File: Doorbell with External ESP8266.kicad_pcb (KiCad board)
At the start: 4 copper layers, 76.2 x 50.8 mm, 29 parts, among them J101 Transformer, J102 To Rectifier, J103 From Rectifier, J104 Button, J105 Chime, K102 Relay, Q101 Q_NMOS_GSD, U101 WeMos_D1_mini, U102 EL817, U104 XC6220B331MR-G

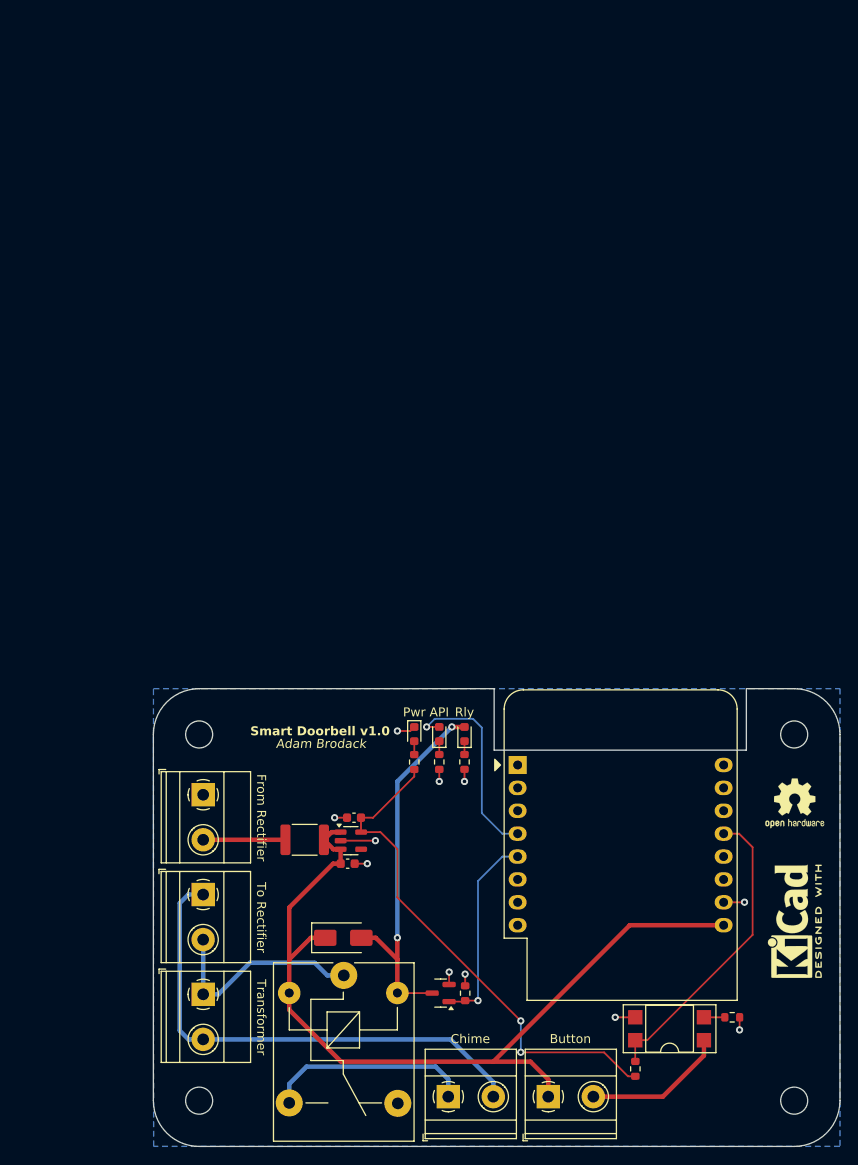
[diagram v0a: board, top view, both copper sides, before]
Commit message: Updated schematic & PCB
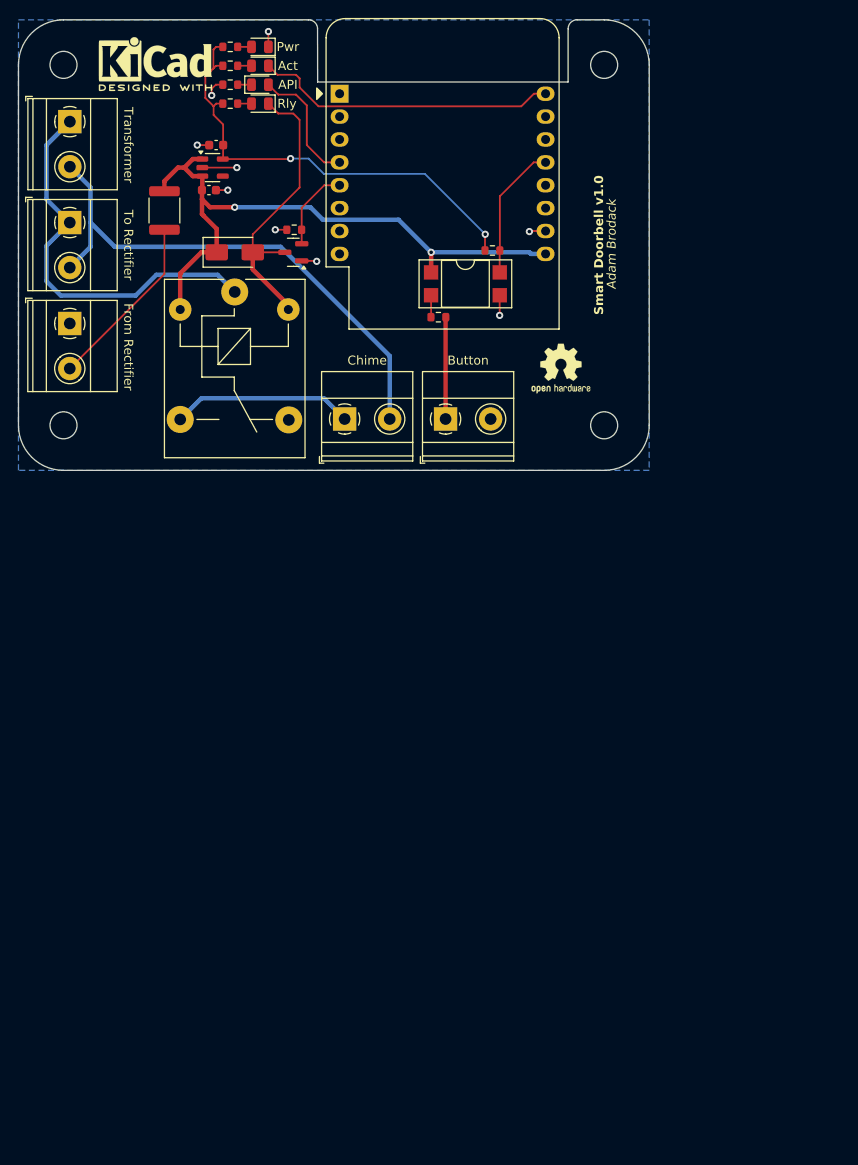
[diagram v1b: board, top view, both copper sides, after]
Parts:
- removed C105: 22uF, Capacitor_SMD:C_0603_1608Metric
- removed C106: 4.7uF, Capacitor_SMD:C_0603_1608Metric
- removed D106: Yellow, LED_SMD:LED_0603_1608Metric
- removed K102: Relay, Relay_THT:Relay_SPDT_SANYOU_SRD_Series_Form_C
- removed R108: 10K, Resistor_SMD:R_0603_1608Metric
- removed U104: XC6220B331MR-G, Package_TO_SOT_SMD:SOT-23-5
- added C101: 22uF, Capacitor_SMD:C_0603_1608Metric, F.Cu at (41.1, 38.9)
- added C102: 4.7uF, Capacitor_SMD:C_0603_1608Metric, F.Cu at (41.9, 33.9)
- added D102: Green, LED_SMD:LED_0805_2012Metric, F.Cu at (46.8, 27.2)
- added D103: Yellow, LED_SMD:LED_0805_2012Metric, F.Cu at (46.8, 25.1)
- added K101: Relay, Relay_THT:Relay_SPDT_SANYOU_SRD_Series_Form_C, F.Cu at (44.0, 50.2)
- added R105: 10K, Resistor_SMD:R_0603_1608Metric, F.Cu at (50.6, 43.3)
- added R107: 10K, Resistor_SMD:R_0603_1608Metric, F.Cu at (72.6, 45.6)
- added U103: EL817, Package_DIP:DIP-4_W7.62mm_SMDSocket_SmallPads, F.Cu at (69.6, 49.3)
- D101: value D_Small -> Red; footprint Diode_SMD:D_SMA -> LED_SMD:LED_0805_2012Metric
- D104: value Red -> White; footprint LED_SMD:LED_0603_1608Metric -> LED_SMD:LED_0805_2012Metric
- D105: value Green -> D_Small; footprint LED_SMD:LED_0603_1608Metric -> Diode_SMD:D_SMA
- J102: value To Rectifier -> From Rectifier
- J103: value From Rectifier -> To Rectifier
- J104: value Button -> Chime
- J105: value Chime -> Button
- R104: value 10K -> 1K
- U102: value EL817 -> XC6220B331MR-G; footprint Package_DIP:DIP-4_W7.62mm_SMDSocket_SmallPads -> Package_TO_SOT_SMD:SOT-23-5
- moved REF** 118.7 mm to (35.2, 24.9), turned to 0 degrees
- moved U102 108.2 mm to (41.5, 36.4), turned to 0 degrees
- moved R104 102.1 mm to (43.5, 29.3), turned to 180 degrees
- moved D101 99.3 mm to (46.8, 23.0), turned to 180 degrees
- moved J101 98.0 mm to (25.7, 31.3)
- moved R106 84.3 mm to (66.6, 53.0), turned to 180 degrees
- moved Q101 83.8 mm to (50.5, 45.8)
- moved R101 82.0 mm to (43.5, 23.0), turned to 180 degrees
- moved R103 81.5 mm to (43.5, 25.1), turned to 180 degrees
- moved R102 78.7 mm to (43.5, 27.2), turned to 0 degrees
- moved J104 78.5 mm to (56.2, 64.3)
- moved H104 77.9 mm to (85.0, 65.0)
- moved H102 77.2 mm to (85.0, 25.0)
- moved U101 77.1 mm to (55.6, 28.2)
- moved H103 76.4 mm to (25.0, 65.0)
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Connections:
- D101 pad 1: VCC -> GND
- D101 pad 2: /RELAY_LED -> Net-(D101-A)
- D104 pad 1: GND -> /RELAY_LED
- D105 pad 1: Net-(D105-K) -> VCC
- D105 pad 2: /HA_STATUS -> /RELAY_LED
- F101 pad 1: Net-(J103-Pin_2) -> Net-(J102-Pin_2)
- J102 pad 1: /AC_B -> GND
- J102 pad 2: /AC_A -> Net-(J102-Pin_2)
- J103 pad 1: GND -> /AC_A
- J103 pad 2: Net-(J103-Pin_2) -> /AC_B
- J104 pad 1: VCC -> Net-(J104-Pin_1)
- J104 pad 2: Net-(J104-Pin_2) -> /AC_B
- J105 pad 2: /AC_B -> GND
- Q101 pad 1: /CHIME -> GND
- Q101 pad 2: GND -> /CHIME
- R101 pad 1: Net-(D104-A) -> Net-(D101-A)
- R102 pad 2: Net-(D105-K) -> Net-(D102-K)
- R103 pad 1: GND -> Net-(D103-A)
- R103 pad 2: Net-(D106-K) -> +3V3
- R104 pad 1: /CHIME -> Net-(D104-A)
- R104 pad 2: GND -> +3V3
- R106 pad 1: Net-(R106-Pad1) -> Net-(J105-Pin_1)
- R106 pad 2: GND -> Net-(R106-Pad2)
- U101 pad 16: unconnected-(U101-TX-Pad16) -> /ESP_TX
- U102 pad 1: Net-(J104-Pin_2) -> VCC
- U102 pad 2: Net-(R106-Pad1) -> GND
- U102 pad 3: GND -> VCC
- U102 pad 4: /DB_BUTTON -> unconnected-(U102-NC-Pad4)
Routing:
- net /ESP_TX: track 0.00 -> 33.8 mm
- net VCC: track 95.9 -> 69.8 mm, vias 0 -> 2
- net /AC_A: track 23.7 -> 44.2 mm
- net Net-(J104-Pin_1): track 0.00 -> 20.2 mm
- net Net-(J102-Pin_2): track 0.00 -> 19.8 mm
- net /DB_BUTTON: track 33.8 -> 15.1 mm
- net Net-(J104-Pin_2): track 15.9 -> 0.00 mm
- net /CHIME: track 22.1 -> 9.24 mm, vias 1 -> 0
- net Net-(J105-Pin_1): track 23.1 -> 11.3 mm
- net /RELAY_LED: track 42.3 -> 32.6 mm, vias 2 -> 0
- net Net-(J103-Pin_2): track 9.12 -> 0.00 mm
- net /HA_STATUS: track 22.7 -> 14.1 mm, vias 1 -> 0
- net +3V3: track 57.0 -> 51.3 mm
- net /AC_B: track 55.9 -> 59.4 mm
- net GND: track 20.0 -> 17.4 mm, vias 11 -> 9
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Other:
- board size 76.2 x 50.8 mm -> 70 x 50 mm
- board text added: "Act"
